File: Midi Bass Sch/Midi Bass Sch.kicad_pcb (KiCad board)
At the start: 2 copper layers, 161.9 x 116.8 mm, 104 parts, among them J10 A SLAVE ISCP, J11 A Slave OUT, J12 D SLAVE ISCP, J13 D Slave OUT, J14 G SLAVE ISCP, J15 G Slave OUT, J16 Power In, J2 Master ISCP, J3 E SLAVE ISCP, J4 E Slave Out, J6 Pluck ISCP, J7 Pick Unit, J8 Pluck Out, SW2 Master Reset, SW3 E-slave Reset, SW4 A-slave Reset, SW5 D-slave Reset, SW6 G-slave Reset, U1 PIC16F1788, U10 PIC16F1789, U16 LM1117MP-1.8, U2 PIC16F1789, U3 PIC16F1789, U8 PIC16F1789, U9 PIC16F1789

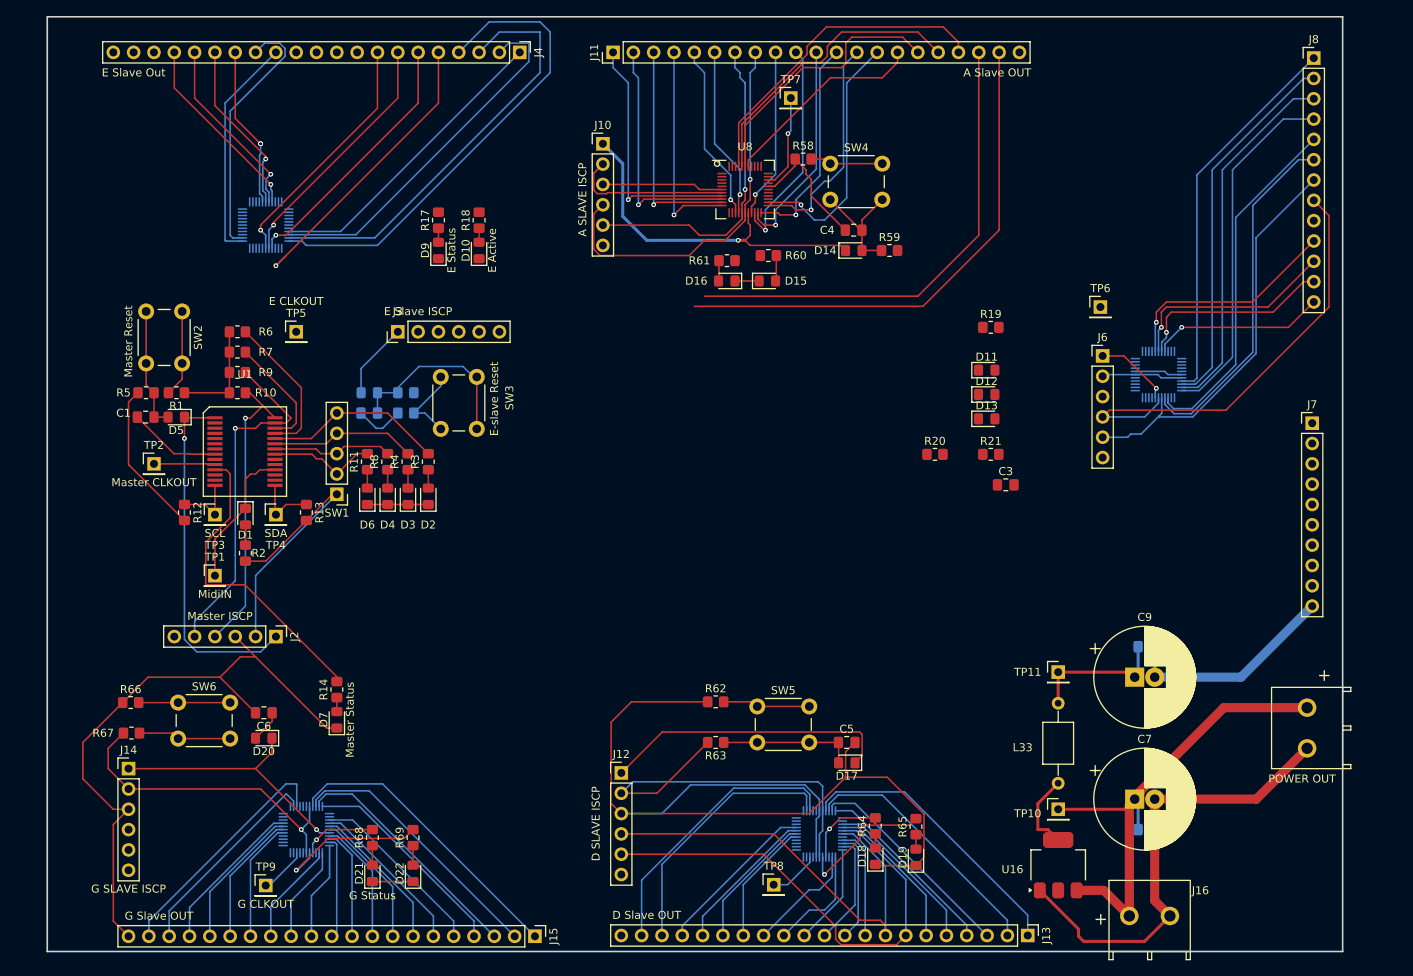
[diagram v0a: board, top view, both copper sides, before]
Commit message: working in finishing Rev A pcb for motherboard
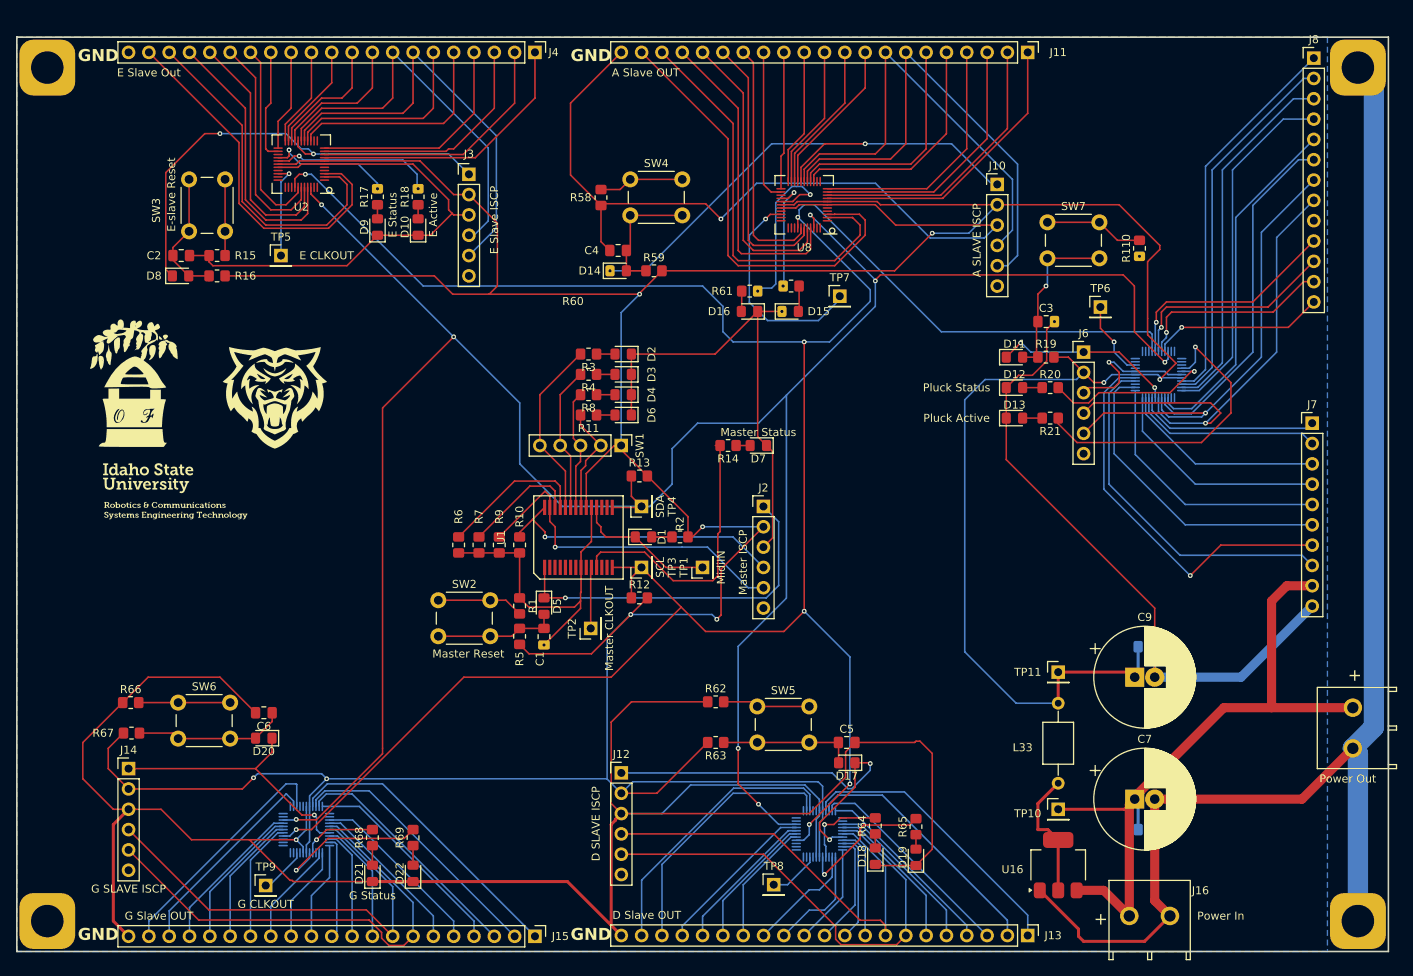
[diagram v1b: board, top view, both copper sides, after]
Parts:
- removed POWER OUT: Two_Pin_Screw_Terminal, OF Footprints:Two_Pin_Screw_Terminal
- added ?: , , F.Cu at (253.4, 112.4)
- added ?: , , F.Cu at (89.5, 112.4)
- added ?: , , F.Cu at (253.4, 219.1)
- added G***: LOGO, Logos:Wisteria Logo .75x.75, F.Cu at (100.5, 151.8)
- added G***: LOGO, Logos:ISU 1inch, F.Cu at (102.5, 165.3)
- added G***: LOGO, Logos:Bengal Head .5x.5, F.Cu at (118.0, 153.7)
- added Power Out: Two_Pin_Screw_Terminal, OF Footprints:Two_Pin_Screw_Terminal, F.Cu at (252.7, 194.9)
- added R110: 10Ω, Resistor_SMD:R_0805_2012Metric_Pad1.20x1.40mm_HandSolder, F.Cu at (226.1, 135.0)
- added REF**: 6-32 Mount, OF Footprints:6-32 Mount, F.Cu at (89.5, 219.1)
- added SW7: Pluck Reset, Button_Switch_THT:SW_PUSH_6mm_H5mm, F.Cu at (214.6, 131.7)
- C2, D8, R15, R16, U2: moved to F.Cu
- moved J2 63.1 mm to (179.1, 167.3), turned to 0 degrees
- moved D7 62.9 mm to (178.4, 159.6), turned to 180 degrees
- moved TP1 61.0 mm to (171.4, 174.9), turned to 90 degrees
- moved TP2 58.3 mm to (157.5, 182.5), turned to 90 degrees
- moved R12 57.9 mm to (163.5, 178.7), turned to 0 degrees
- moved R14 57.6 mm to (174.6, 159.6), turned to 180 degrees
- moved C1 56.9 mm to (151.6, 183.5), turned to -90 degrees
- moved R5 55.8 mm to (148.6, 183.5), turned to -90 degrees
- moved R2 54.4 mm to (168.6, 171.1), turned to 0 degrees
- moved TP3 53.7 mm to (163.8, 174.9), turned to 90 degrees
- moved J11 51.8 mm to (212.1, 110.5), turned to -90 degrees
- moved D5 51.7 mm to (151.6, 179.7), turned to -90 degrees
- moved R1 50.5 mm to (148.6, 179.7), turned to -90 degrees
- moved D1 49.8 mm to (164.1, 171.1), turned to 0 degrees
- moved J10 49.6 mm to (208.3, 127.0)
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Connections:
- J15 pad 7: RB6 A -> RB6 G
- J15 pad 8: RB7 A -> RB7 G
- U10 pad 16: RB6 A -> RB6 G
- U10 pad 17: RB7 A -> RB7 G
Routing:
- net +5v: track 191.5 -> 561.5 mm, vias 1 -> 9
- net GND: track 308.7 -> 654.5 mm, vias 0 -> 3
- net I2Cclk: track 8.00 -> 318.0 mm, vias 0 -> 7
- net I2Cdat: track 8.05 -> 307.7 mm, vias 0 -> 8
- net Earth_GND: track 61.6 -> 176.2 mm
- net RB6 G: track 0.00 -> 60.0 mm
- net RB7 G: track 0.00 -> 55.6 mm
- net Net-(U3-RE2/AN7/PSMC3A): track 0.00 -> 48.8 mm, vias 0 -> 1
- net MSCLR E: track 9.52 -> 58.3 mm, vias 0 -> 2
- net C3: track 0.00 -> 46.7 mm
- net Net-(U3-RE1/AN6/PSMC3B): track 0.00 -> 44.9 mm
- net B2: track 0.00 -> 43.5 mm
- net Net-(U3-RA5/AN4/C2OUT/OPA1IN+): track 0.00 -> 39.0 mm
- net Net-(U3-RD6/PSMC3D): track 0.00 -> 38.8 mm, vias 0 -> 1
- net Net-(U3-RA4/C1OUT/OPA1IN+/T0CKI): track 0.00 -> 32.7 mm
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- added copper zone on B.Cu, net GND
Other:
- board size 161.9 x 116.8 mm -> 171.5 x 114.3 mm
- board text added: "GND"
